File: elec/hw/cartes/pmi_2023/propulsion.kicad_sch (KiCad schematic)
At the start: 55 parts, among them U1 DRV8231ADDAR, U2 SN74LVC1T45DBV, U3 SN74LVC1T45DBV, U4 DRV8231ADDAR, U5 SN74LVC1T45DBV, U6 SN74LVC1T45DBV, U7 SN74LVC1T45DBV

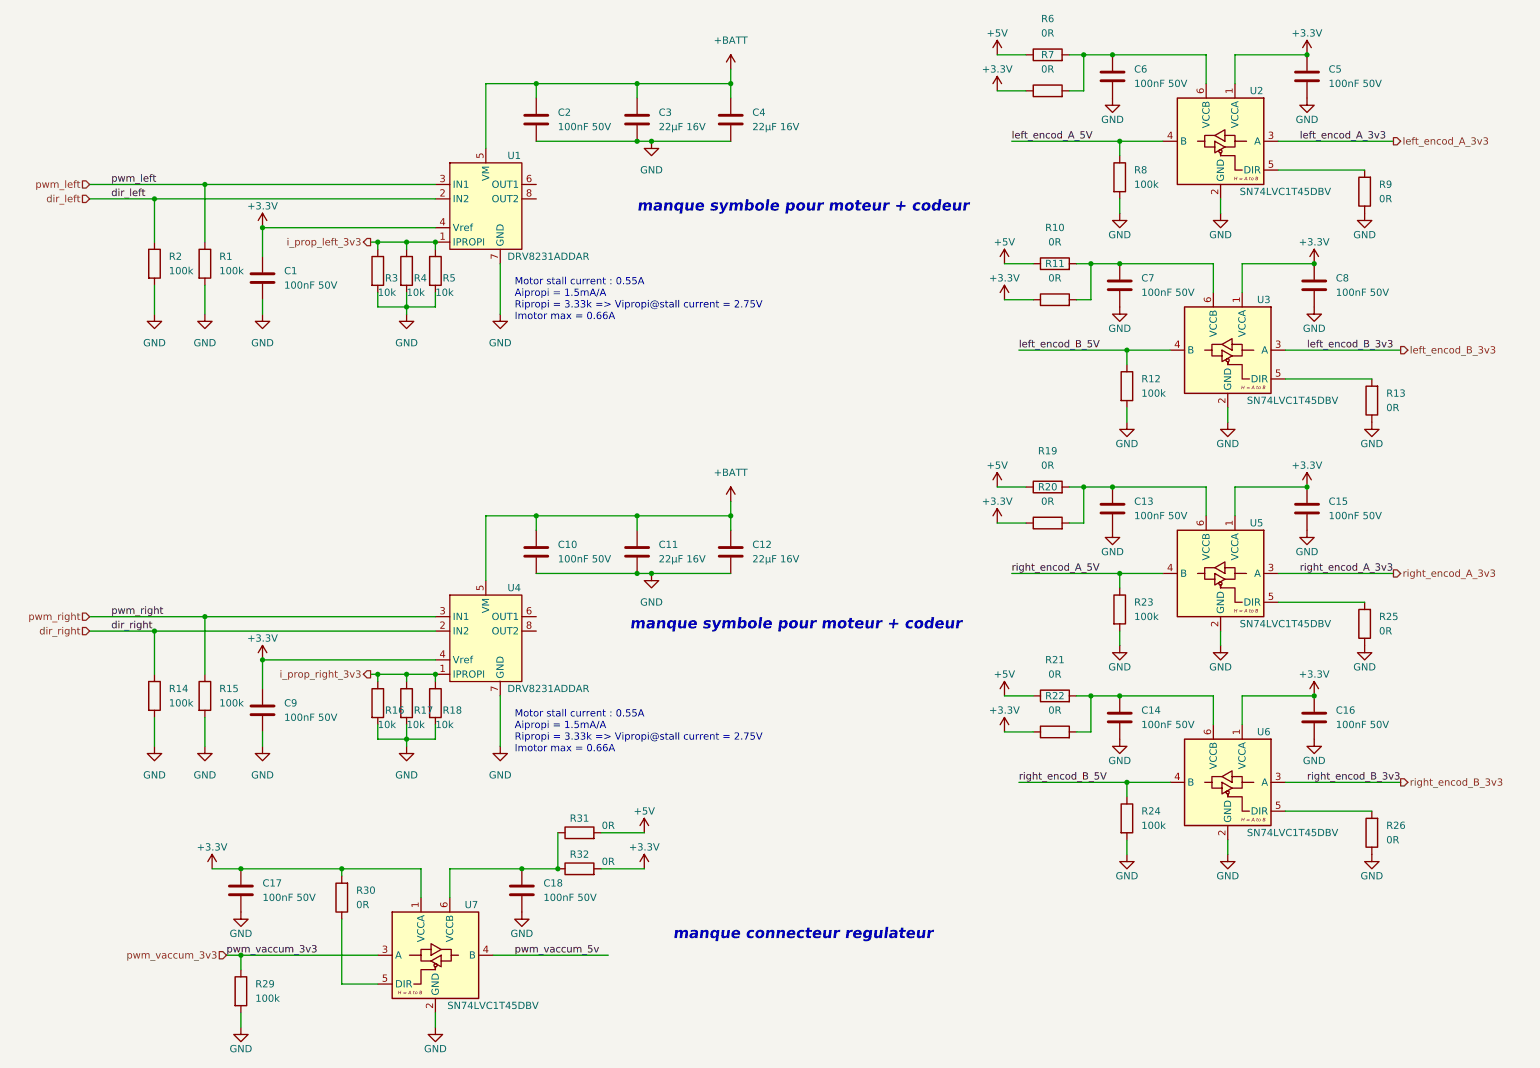
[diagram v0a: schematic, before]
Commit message: pmi2023 wip
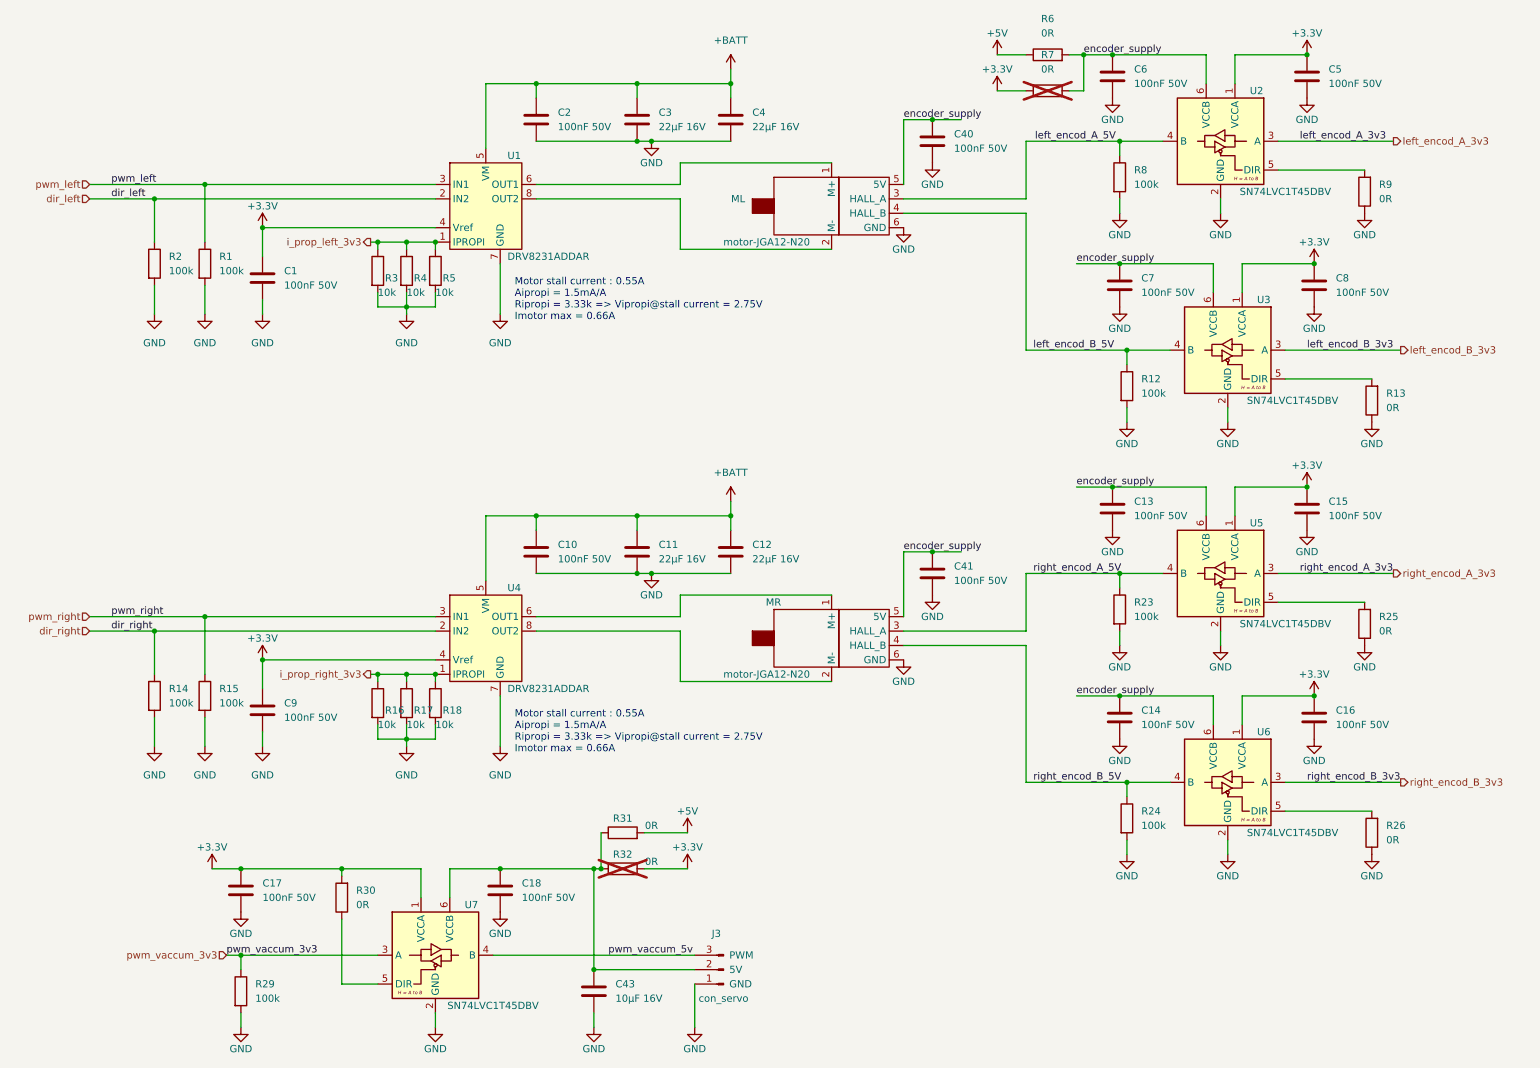
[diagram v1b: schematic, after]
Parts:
- removed R10, R11, R19, R20, R21, R22: 0R, cocotter_resistor:r0603_reflow, symbol cocotter_resistors:R_0R_0603
- added C40, C41: 100nF 50V, symbol cocotter_capacitors:C_100nF_50V_0603
- added C43: 10µF 16V, symbol cocotter_capacitors:C_10µF_16V_0805
- added J3: con_servo, symbol cocotter_connectors:con_servo
- added ML, MR: motor-JGA12-N20, symbol cocotter_connectors:motor-JGA12-N20
- R32, R7: now not fitted
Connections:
- net GND: now also C40.2, C41.2, C43.2, J3.1 (GND), ML.6 (GND), MR.6 (GND)
- net left_encod_A_5V: now also ML.3 (HALL_A)
- net left_encod_B_5V: now also ML.4 (HALL_B)
- net pwm_vaccum_5v: now also J3.3 (PWM)
- net right_encod_A_5V: now also MR.3 (HALL_A)
- net right_encod_B_5V: now also MR.4 (HALL_B)
- net encoder_supply: now reaches C14.1, U6.6 (VCCB)
- net encoder_supply: now also C13.1, C6.1, C7.1, R6.2, R7.2, U2.6 (VCCB), U3.6 (VCCB), U5.6 (VCCB), C40.1, C41.1, ML.5 (5V), MR.5 (5V)
- net at C18.1, R31.1, R32.1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: now also C43.1, J3.2 (5V)
- net at U1.6 (OUT1): now also ML.1 (M+)
- net at U1.8 (OUT2): now also ML.2 (M-)
- net at U4.6 (OUT1): now also MR.1 (M+)
- net at U4.8 (OUT2): now also MR.2 (M-)
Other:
- note removed: "manque connecteur regulateur"
- note removed: "manque symbole pour moteur + codeur"
- moved on the sheet: C18, R31
